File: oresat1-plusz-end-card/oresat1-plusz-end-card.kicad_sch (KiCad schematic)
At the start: 35 parts, among them J1 J-SAMTEC-TFM-120-01-L-D-RA, J2 M55-7101242R, J3 M55-7101242R, J4 M55-7101242R, J5 M55-7101242R, J6 U.FL-R-SMT-1

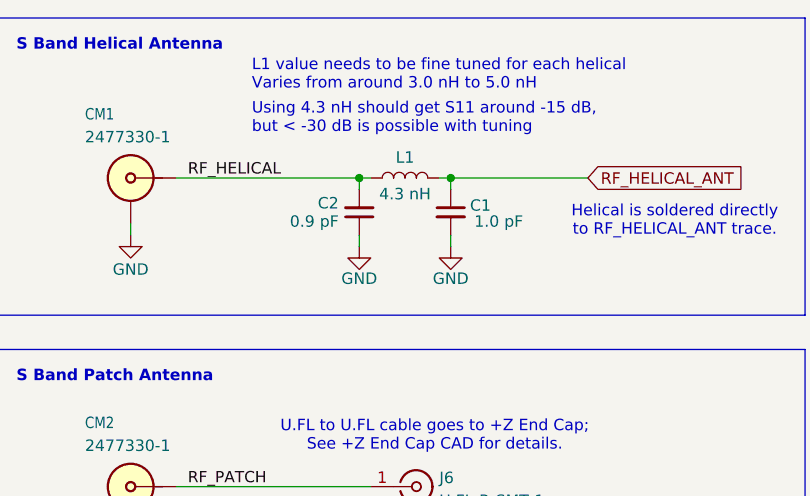
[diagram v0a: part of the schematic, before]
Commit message: Polishing schematic, syncing, polishing layout, added releases folder, updating makefile
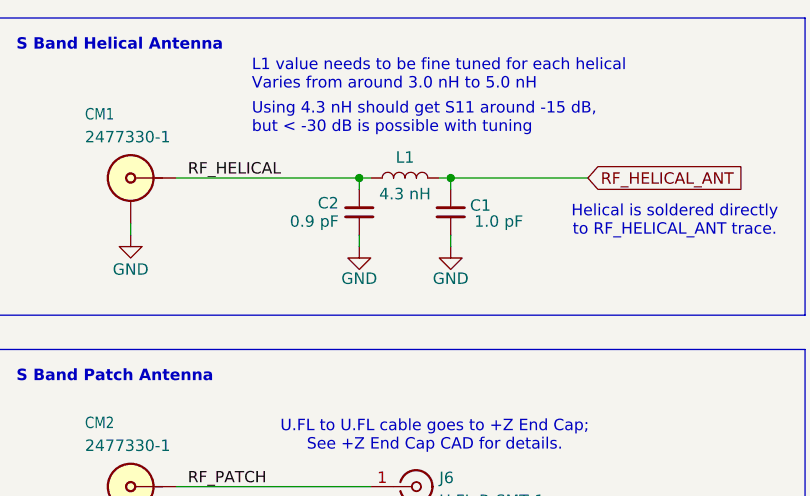
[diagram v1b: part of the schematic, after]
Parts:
- HW10, HW11, HW12, HW13, HW14, HW4, HW9: DIS McMaster-Carr -> McMaster Carr
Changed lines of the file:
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@@
 			)
 		)
-		(property "DIS" "McMaster-Carr"
+		(property "DIS" "McMaster Carr"
 			(at 248.92 254 0)
 			(hide yes)
@@
 			)
 		)
-		(property "DIS" "McMaster-Carr"
+		(property "DIS" "McMaster Carr"
 			(at 278.13 238.76 0)
 			(hide yes)
@@
 			)
 		)
-		(property "DIS" "McMaster-Carr"
+		(property "DIS" "McMaster Carr"
 			(at 248.92 238.76 0)
 			(hide yes)
@@
 			)
 		)
-		(property "DIS" "McMaster-Carr"
+		(property "DIS" "McMaster Carr"
 			(at 278.13 246.38 0)
 			(hide yes)
@@
 			)
 		)
-		(property "DIS" "McMaster-Carr"
+		(property "DIS" "McMaster Carr"
 			(at 278.13 231.14 0)
 			(hide yes)
@@
 			)
 		)
-		(property "DIS" "McMaster-Carr"
+		(property "DIS" "McMaster Carr"
 			(at 248.92 231.14 0)
 			(hide yes)
@@
 			)
 		)
-		(property "DIS" "McMaster-Carr"
+		(property "DIS" "McMaster Carr"
 			(at 248.92 246.38 0)
 			(hide yes)
